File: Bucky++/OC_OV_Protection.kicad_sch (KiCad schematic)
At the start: 65 parts, among them IC10 TPS259830ONRGER, IC7 TPS259830ONRGER, IC8 TPS259830ONRGER, IC9 TPS259830ONRGER, Q9 RS1E260ATTB1, U4 ADM1270ACPZ

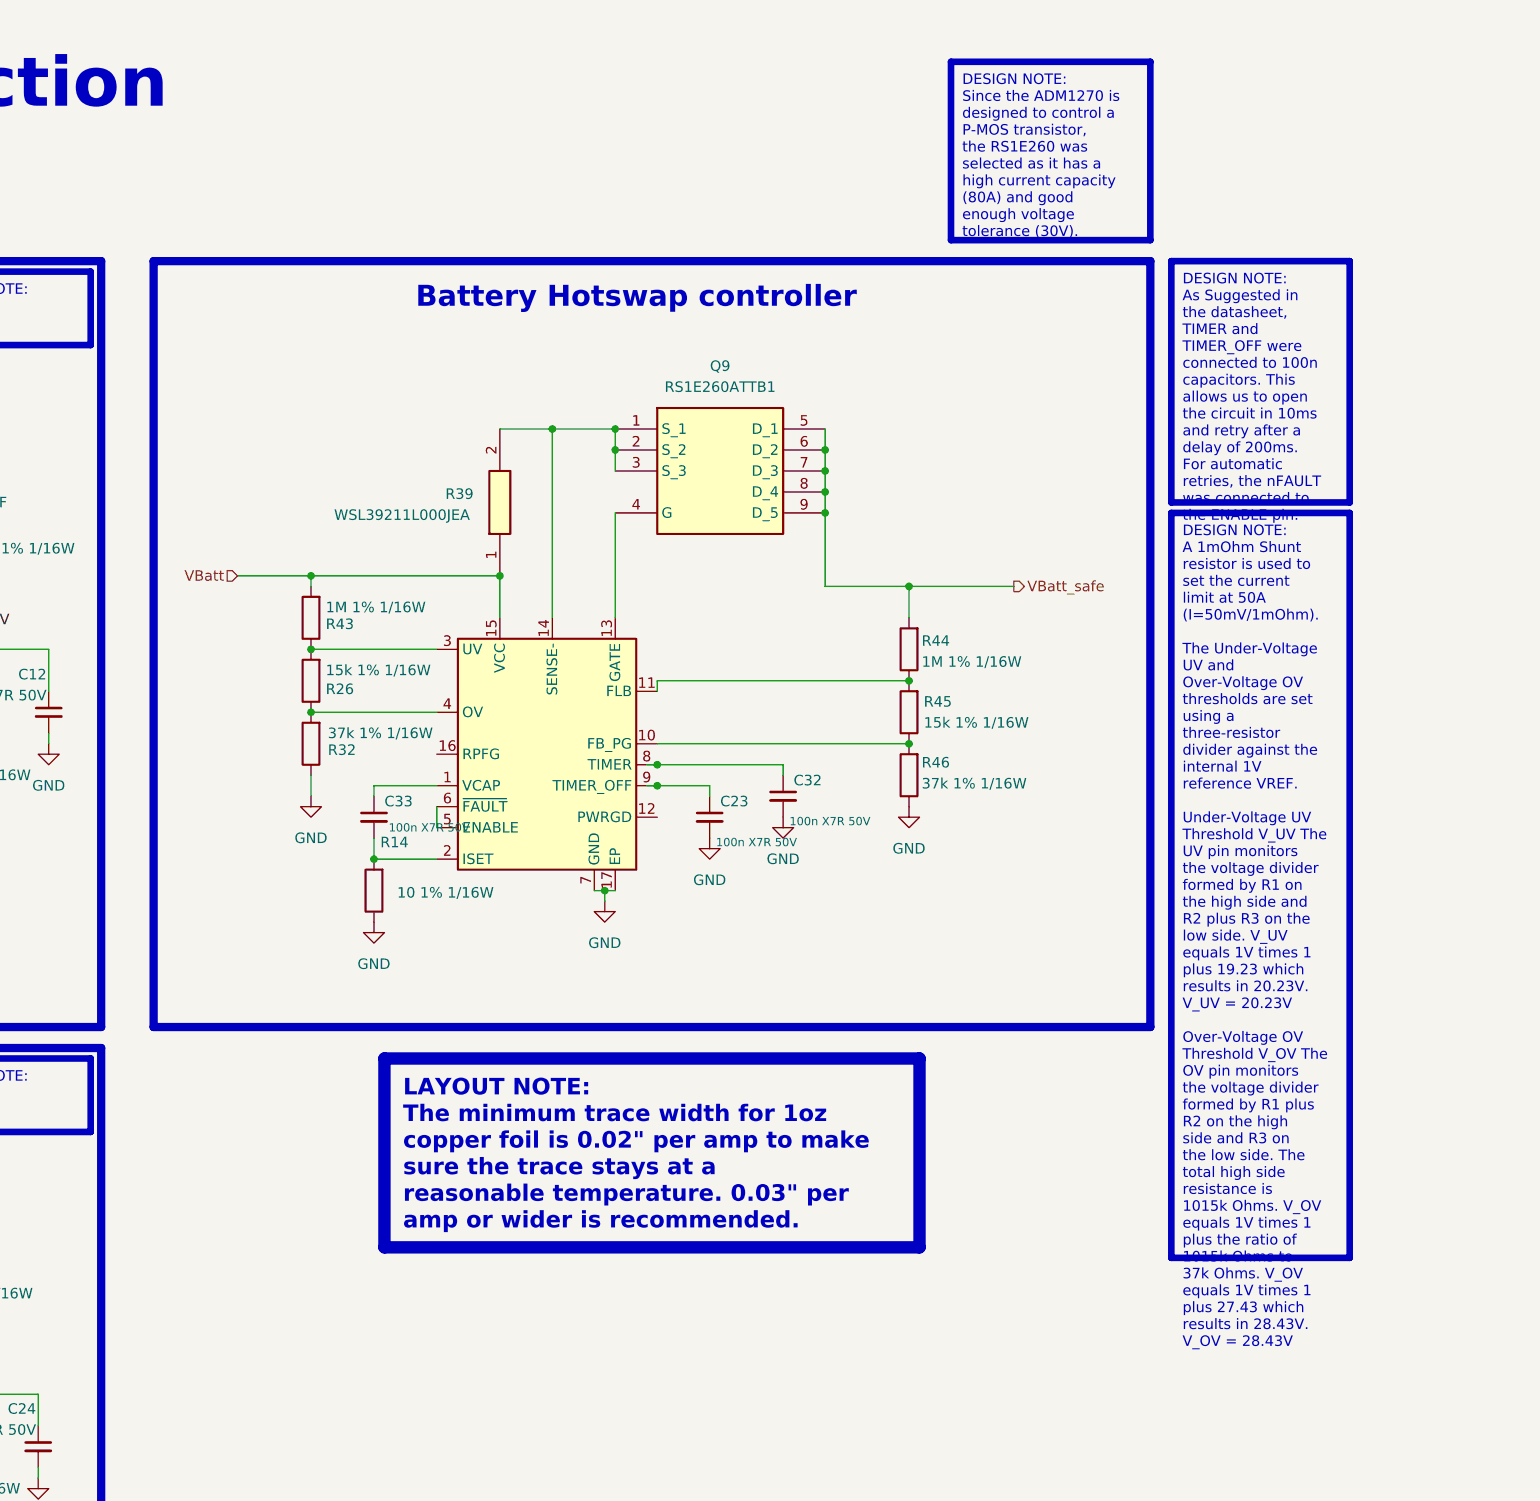
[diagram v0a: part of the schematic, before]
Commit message: implemented foldback
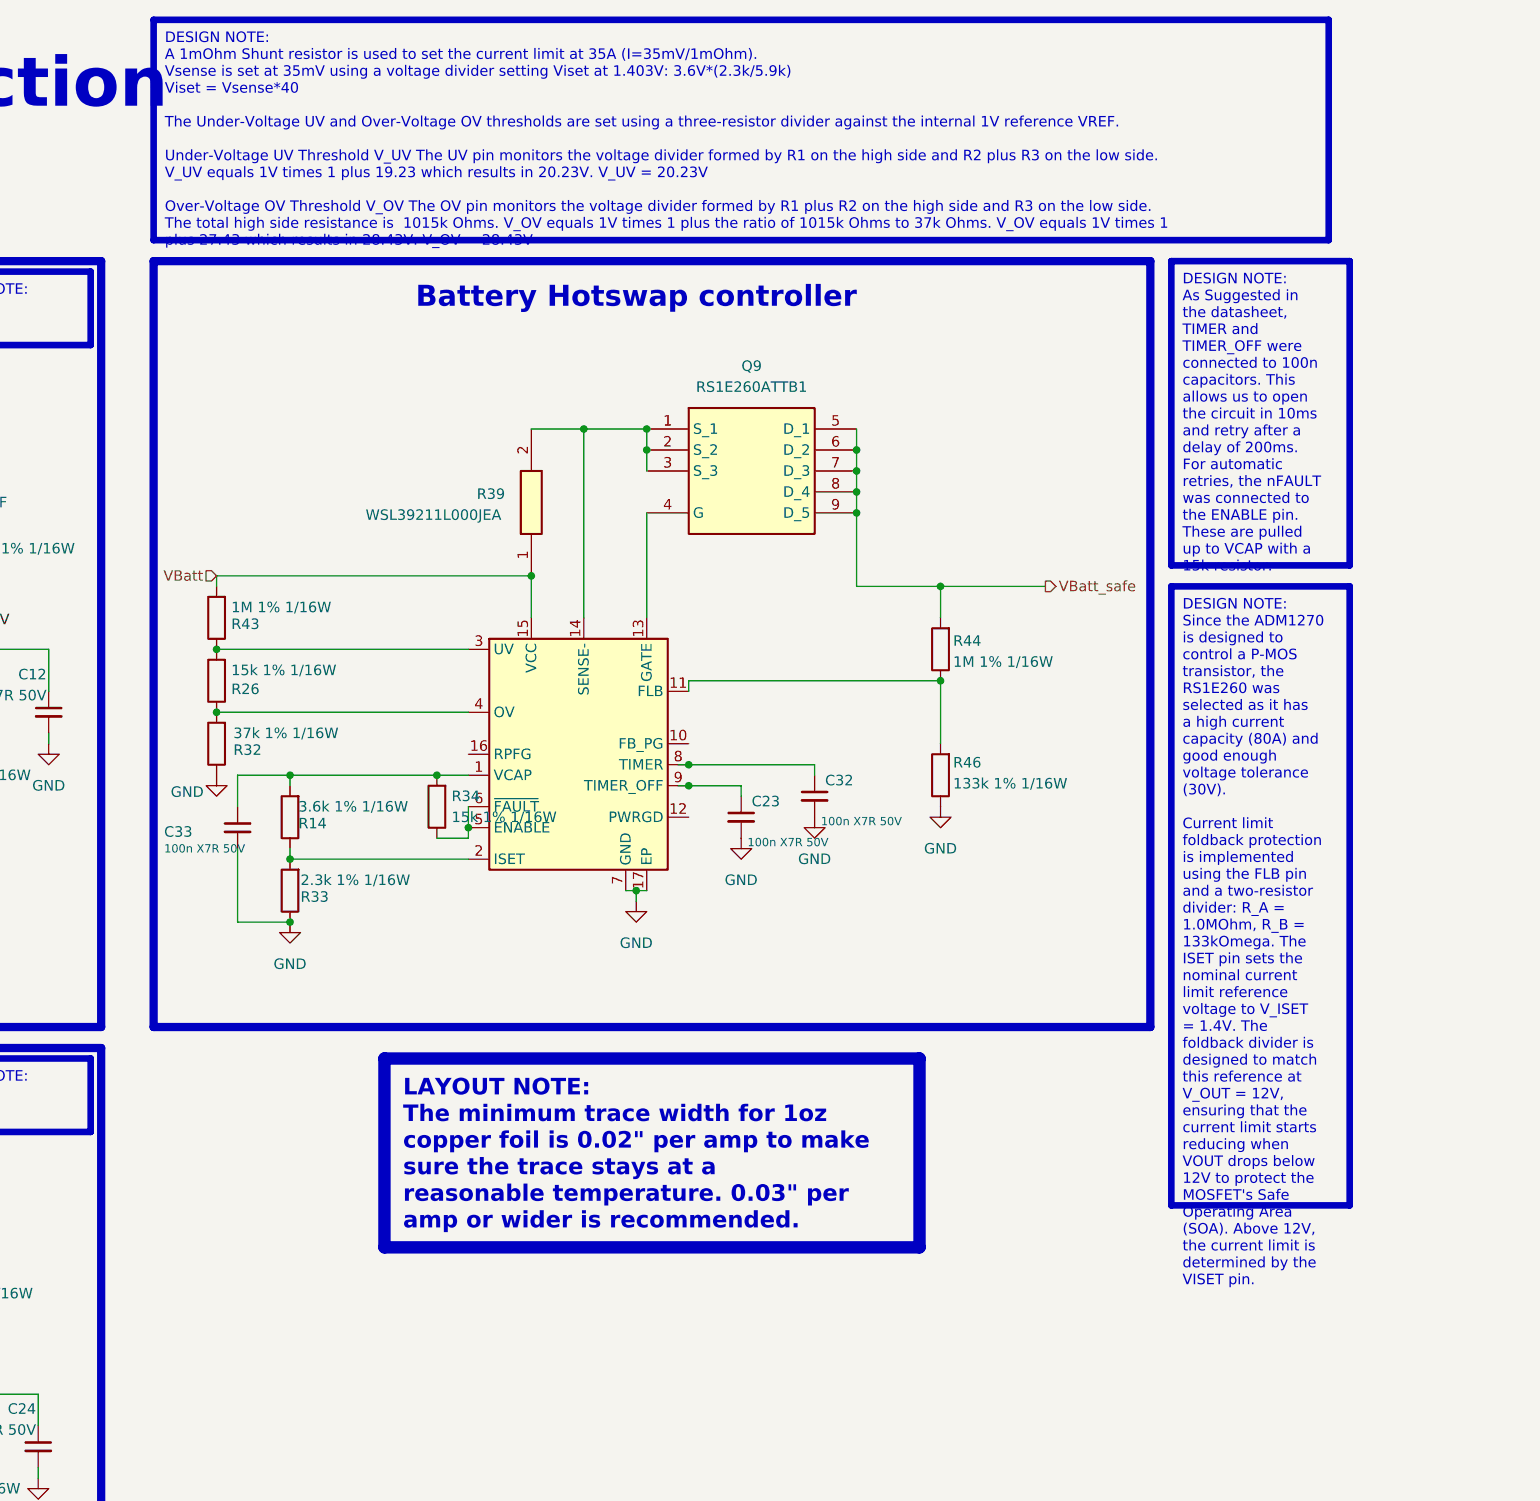
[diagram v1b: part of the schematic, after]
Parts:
- removed R45: 15k 1% 1/16W, 0_resistor_smd:R_0402_1005_DensityHigh, symbol Device:R
- added R33: 2.3k 1% 1/16W, 0_resistor_smd:R_0402_1005_DensityHigh, symbol Device:R
- added R34: 15k 1% 1/16W, 0_resistor_smd:R_0402_1005_DensityHigh, symbol Device:R
- R14: value 10 1% 1/16W -> 3.6k 1% 1/16W
- R46: value 37k 1% 1/16W -> 133k 1% 1/16W
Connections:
- net GND: now also C33.2, R33.1; no longer R14.1
- net at C33.1, U4.1 (VCAP): now also R14.2, R34.2
- net at U4.10 (FB_PG): no longer R46.2
- net at R44.1, U4.11 (FLB): now also R46.2
- net at U4.5 (ENABLE), U4.6 (~{FAULT}): now also R34.1
- new net: R14.1, R33.2, U4.2 (ISET)
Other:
- moved on the sheet: C23, C32, C33, Q9, R26, R32, R39, R43, R44, R46
